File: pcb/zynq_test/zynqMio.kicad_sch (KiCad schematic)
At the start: 31 parts, among them SW201 SW_SPDT, SW202 SW_SPDT, SW203 SW_SPDT, U201 DSC1001CI2-033.3300, U202 XC7Z020-2CLG400I

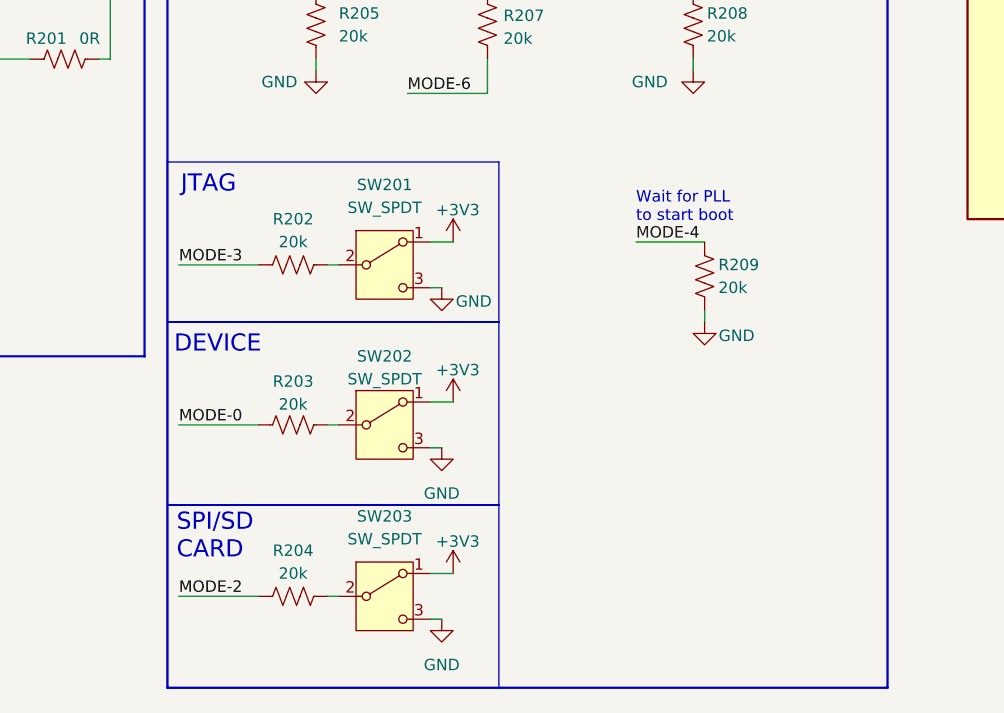
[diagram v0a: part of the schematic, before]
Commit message: Almost done with BOM
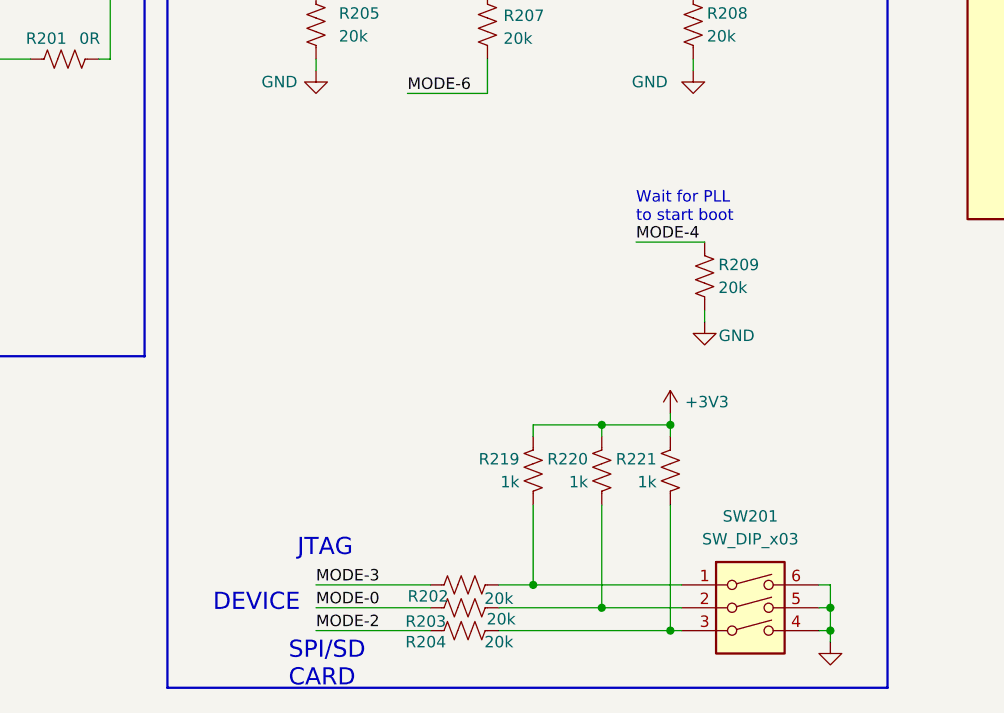
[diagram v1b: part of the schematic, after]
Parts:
- removed SW201, SW202, SW203: SW_SPDT, symbol Switch:SW_SPDT
- added R219, R220, R221: 1k, Resistor_SMD:R_0402_1005Metric, symbol Device:R_US
- added SW201: SW_DIP_x03, Button_Switch_SMD:SW_DIP_SPSTx03_Slide_6.7x9.18mm_W8.61mm_P2.54mm_LowProfile, symbol Switch:SW_DIP_x03
- C202: footprint (none) -> Capacitor_SMD:C_0402_1005Metric
- R201: footprint (none) -> Resistor_SMD:R_0402_1005Metric
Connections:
- net +3V3: now also R219.2, R220.2, R221.2
- net GND: now also SW201.4, SW201.5, SW201.6
- net at R202.2: now also R219.1, SW201.1
- net at R204.2: now also R221.1, SW201.3
- net at R203.2: now also R220.1, SW201.2
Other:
- moved on the sheet: R202, R203, R204
